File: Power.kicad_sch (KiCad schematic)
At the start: 33 parts, among them IC1 LM74502HDDFR, IC2 LM74502HDDFR, J6 PowerDebug, Q3 NVMFWS1D7N04XMT1G, Q4 NVMFWS1D7N04XMT1G, Q5 NVMFWS1D7N04XMT1G, Q6 NVMFWS1D7N04XMT1G, U3 LMR33630ADDA

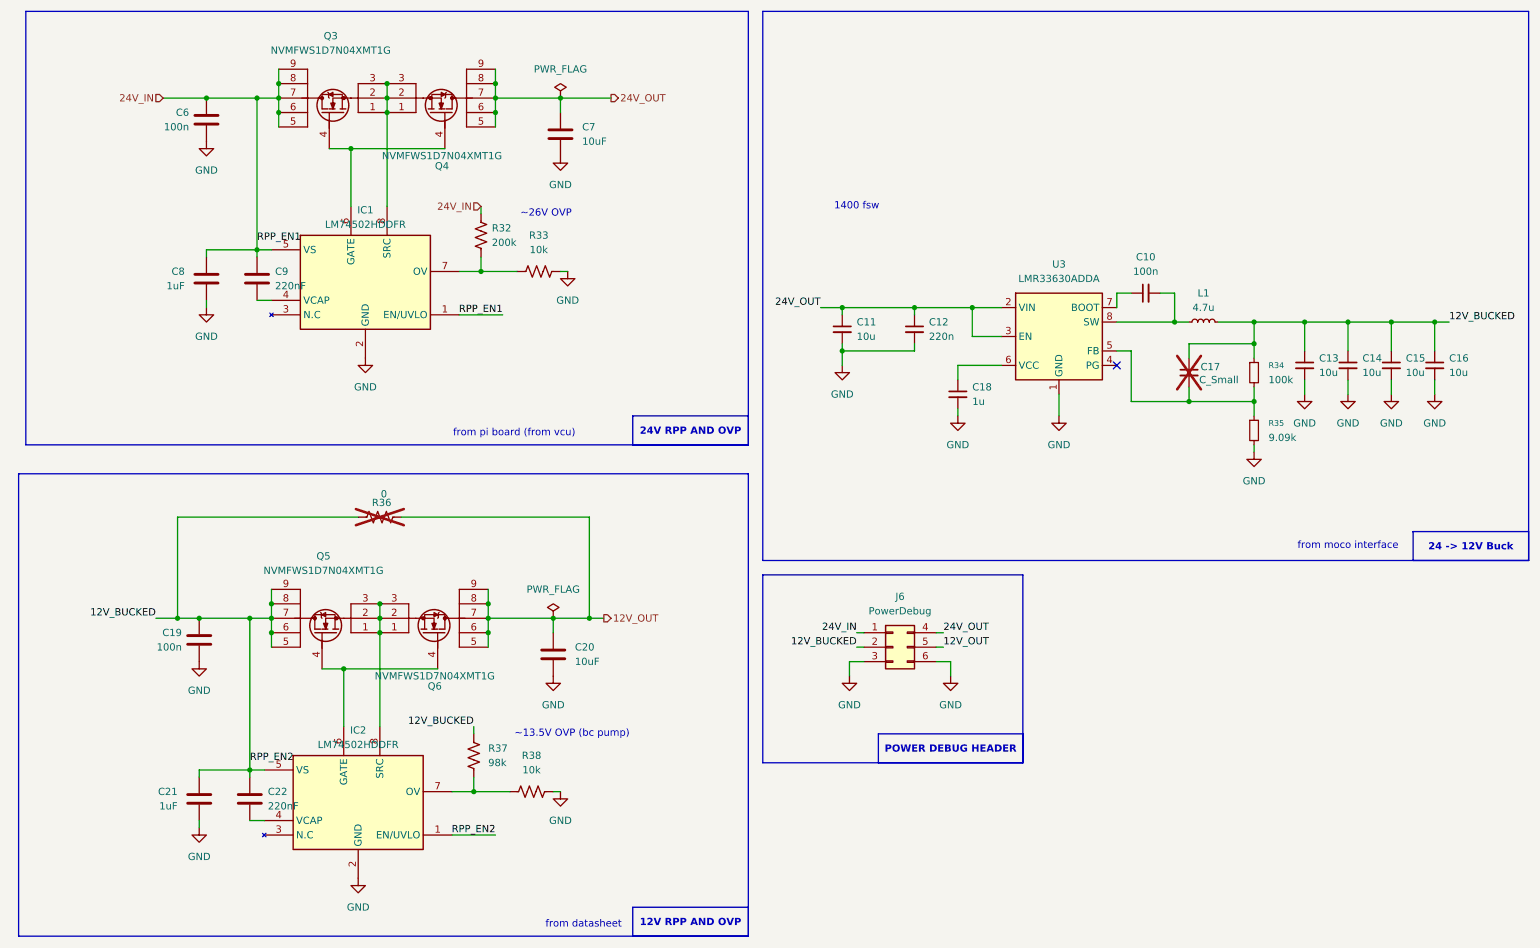
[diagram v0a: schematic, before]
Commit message: lakshays bs
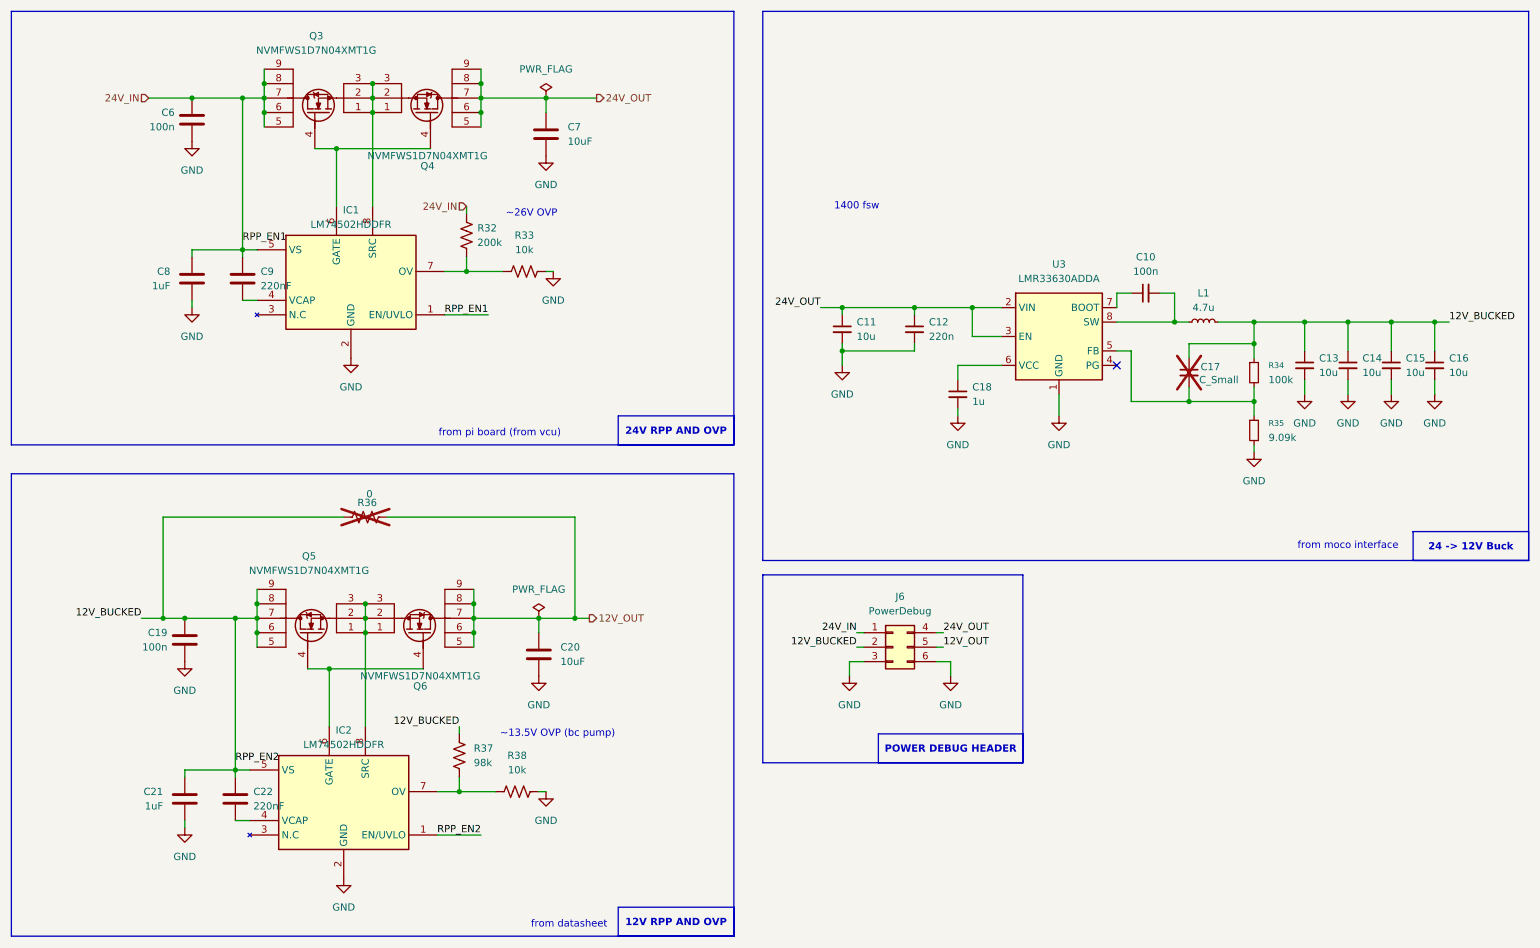
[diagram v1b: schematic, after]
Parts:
- L1: P/N (none) -> CKCS5040
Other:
- moved on the sheet: C19, C20, C21, C22, C6, C7, C8, C9, IC1, IC2, Q3, Q4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
